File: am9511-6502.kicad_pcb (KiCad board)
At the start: 2 copper layers, 84.9 x 67.5 mm, 24 parts, among them J1 Conn_01x18_Pin, U1 AM9511A, U2 GAL16V8, U3 74HC112, U4 ADA-TPS61040, U5 74HC123, X1 4 MHz

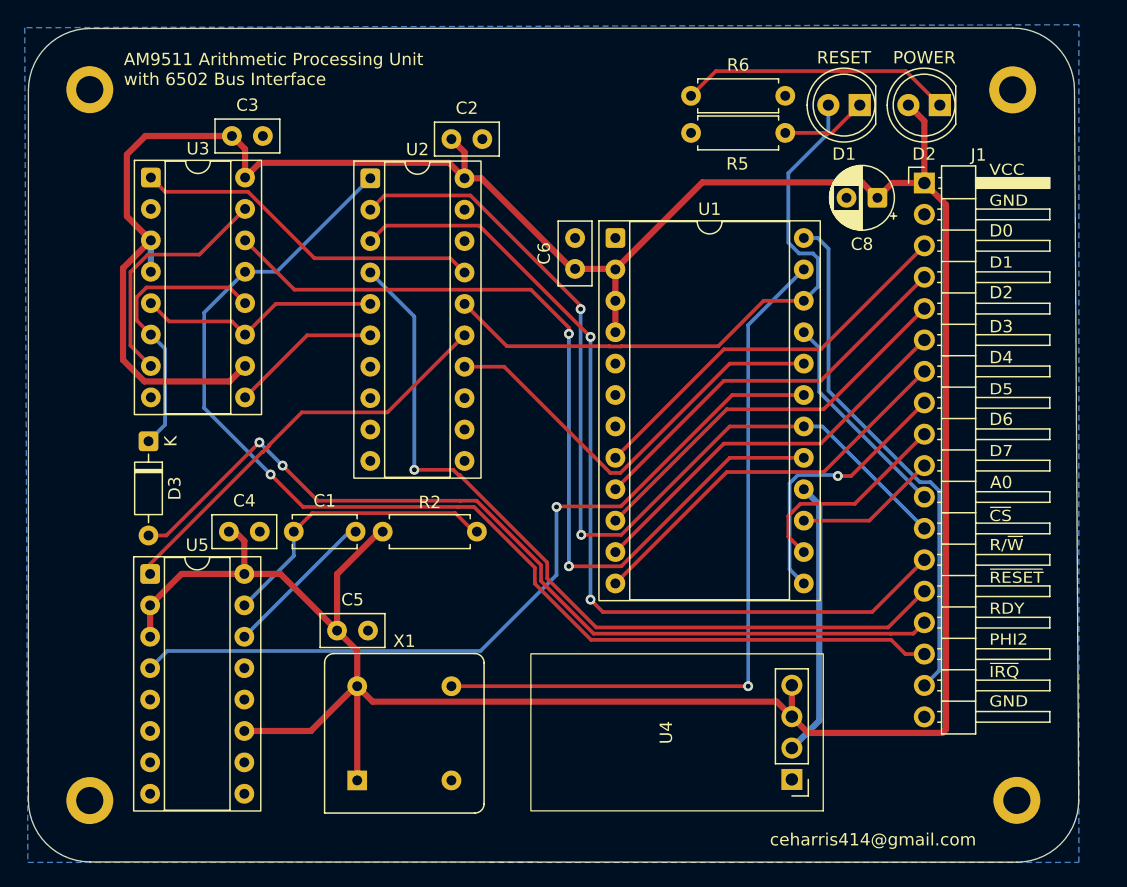
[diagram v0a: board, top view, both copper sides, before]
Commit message: additional PCB cleanup
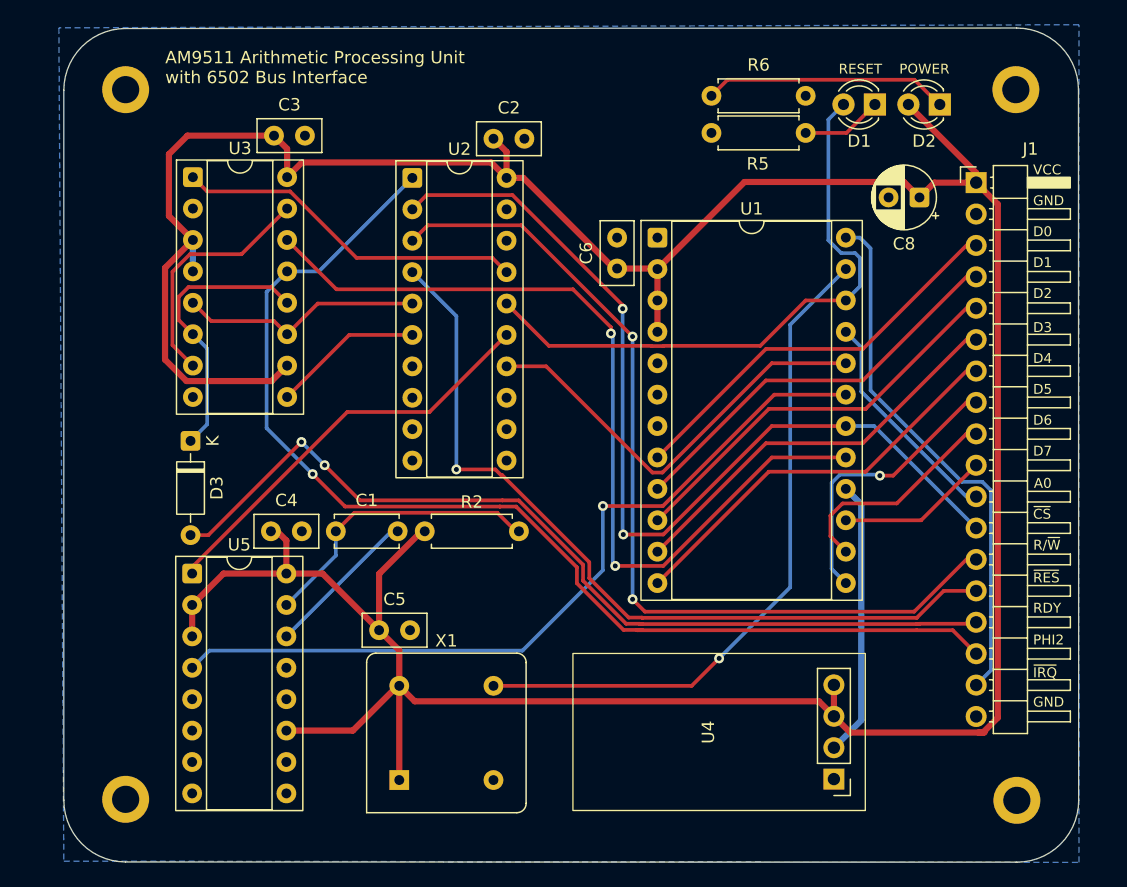
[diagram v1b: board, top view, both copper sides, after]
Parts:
- D1, D2: footprint LED_THT:LED_D5.0mm -> LED_THT:LED_D3.0mm
- J1: footprint Connector_PinHeader_2.54mm:PinHeader_1x18_P2.54mm_Horizontal -> am9511-6502-footprints:PinHeader_1x18_P2.54mm_Horizontal
- U2: value GAL16V8 -> ATF16V8B
- moved J1 4.19 mm to (179.2, 62.5)
- moved C1 3.40 mm to (127.4, 90.7)
- moved C2 3.40 mm to (140.2, 59.0)
- moved C3 3.40 mm to (122.4, 58.7)
- moved C4 3.40 mm to (122.2, 90.7)
- moved C5 3.40 mm to (130.9, 98.7)
- moved C6 3.40 mm to (150.2, 69.5)
- moved D3 3.40 mm to (115.7, 83.4)
- moved R2 3.40 mm to (134.6, 90.7)
- moved U1 3.40 mm to (153.4, 67.0)
- moved U2 3.40 mm to (133.6, 62.1)
- moved U3 3.40 mm to (115.8, 62.1)
- moved U4 3.40 mm to (157.5, 107.0)
- moved U5 3.40 mm to (115.8, 94.1)
- moved X1 3.40 mm to (132.5, 110.8)
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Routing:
- net Net-(U1-CLK): track 59.6 -> 54.9 mm
- net VCC: track 278.6 -> 281.8 mm
- net Net-(D2-K): track 21.7 -> 19.5 mm
- net /~{IRQ}: track 42.4 -> 43.2 mm
- net /~{CS}: track 74.5 -> 75.3 mm
- net /D7: track 11.6 -> 12.4 mm
- net /D6: track 17.2 -> 18.0 mm
- net /D5: track 22.2 -> 23.0 mm
- net /RESET: track 49.7 -> 49.0 mm
- net /PHI2: track 92.9 -> 92.3 mm
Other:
- board size 84.9 x 67.5 mm -> 82.1 x 67.5 mm
- board text added: "~{RES}"
- board text removed: "ceharris414@gmail.com"
- board text removed: "~{RESET}"
